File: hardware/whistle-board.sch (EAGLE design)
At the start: 17 parts, among them IC1 MCP4131, IC2 L272, Q1 BC638, Q3 BC638

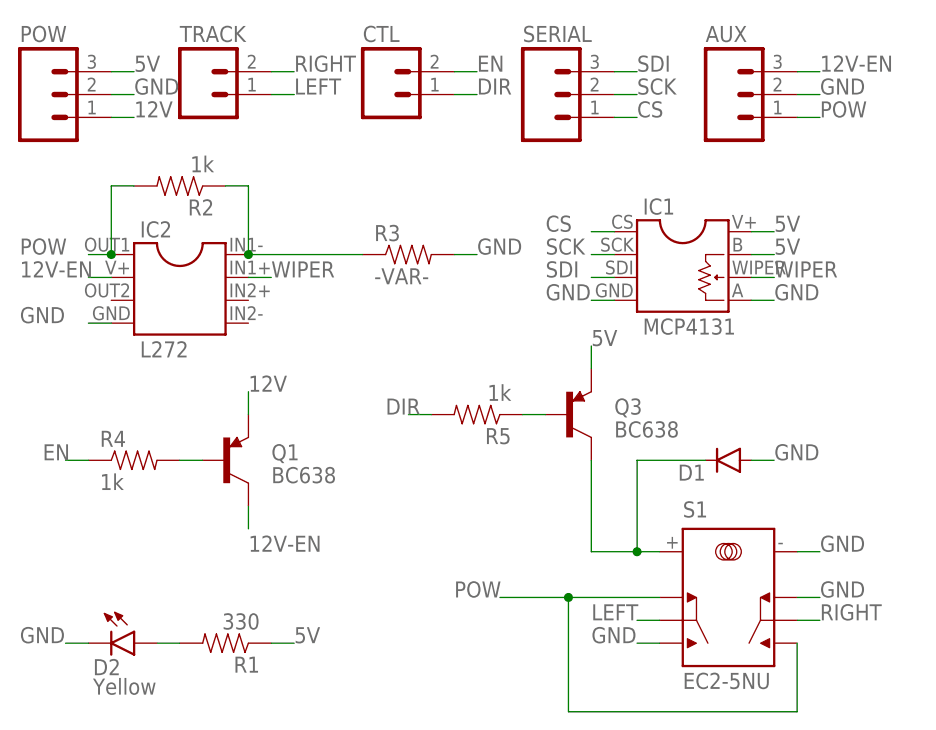
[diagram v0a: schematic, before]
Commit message: revisions after the most recent draft was assembled and tested
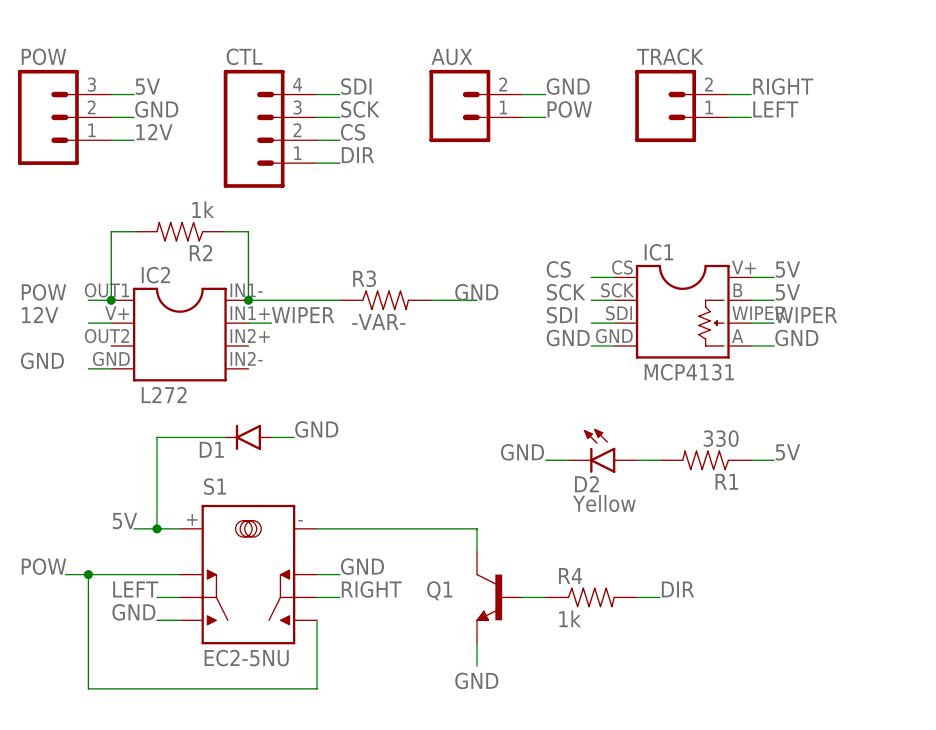
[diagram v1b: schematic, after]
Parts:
- removed Q3: BC638, custom-parts:TRANSISTOR_PNPTO92
- removed R5: 1k, SparkFun-Resistors:1KOHM-1/4W-5%(PTH)
- removed SERIAL: (no value), SparkFun-Connectors:M03PTH
- AUX: device SparkFun-Connectors:M03PTH -> SparkFun-Connectors:M02PTH
- CTL: device SparkFun-Connectors:M02PTH -> SparkFun-Connectors:M04PTH
- Q1: value BC638 -> (none); device custom-parts:TRANSISTOR_PNPTO92 -> custom-parts:TRANSISTOR_NPNTO92
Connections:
- removed net 12V-EN: AUX.3, IC2.V+, Q1.C
- removed net EN: CTL.2, R4.1
- removed net N$5: Q3.B, R5.1
- net 12V: now also IC2.V+; no longer Q1.E
- net 5V: now also D1.C, S1.+; no longer Q3.E
- net CS: now also CTL.2; no longer SERIAL.1
- net DIR: now also R4.2; no longer R5.2
- net GND: now also Q1.E; no longer S1.-
- net N$1: now also Q1.C, S1.-; no longer Q1.B, R4.2
- net N$2: now also Q1.B, R4.1; no longer D1.C, Q3.C, S1.+
- net SCK: now also CTL.3; no longer SERIAL.2
- net SDI: now also CTL.4; no longer SERIAL.3
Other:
- moved on the sheet: D1, D2, IC1, IC2, POW, Q1, R1, R2, R3, R4, S1, TRACK
